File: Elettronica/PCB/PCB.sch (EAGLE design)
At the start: 60 parts, among them IC1 7805TV, J2 455-1750-1-ND, SW2 EC12E_SW

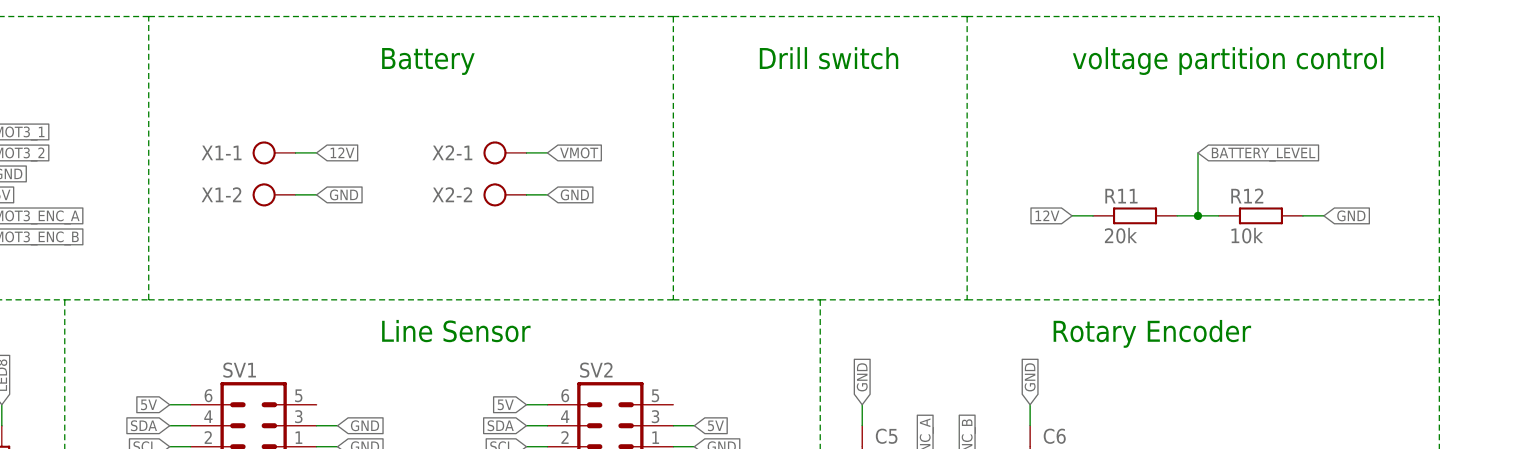
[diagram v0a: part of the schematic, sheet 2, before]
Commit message: PCB schematico
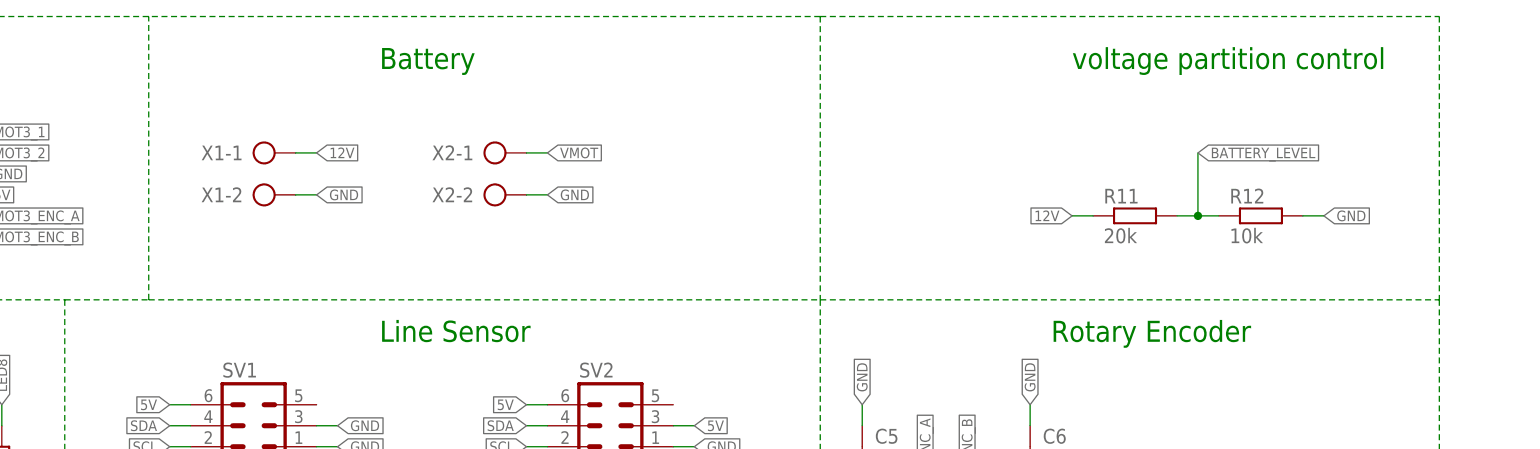
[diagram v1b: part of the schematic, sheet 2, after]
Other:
- note removed: "Drill switch"
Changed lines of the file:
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@@
 <?xml version="1.0" encoding="utf-8"?>
 <!DOCTYPE eagle SYSTEM "eagle.dtd">
-<eagle version="9.3.1">
+<eagle version="9.2.2">
 <drawing>
 <settings>
@@
 <text x="40.64" y="167.64" size="2.54" layer="91">Encoder pin</text>
 <text x="127" y="167.64" size="2.54" layer="91">Battery</text>
-<text x="172.72" y="167.64" size="2.54" layer="91">Drill switch</text>
 <text x="43.18" y="134.62" size="2.54" layer="91">Led</text>
 <text x="121.92" y="109.22" size="1.778" layer="91">ADR-GND
@@
 <wire x1="160.02" y1="5.08" x2="160.02" y2="25.4" width="1.016" layer="91" style="longdash"/>
 <wire x1="160.02" y1="25.4" x2="255.27" y2="25.4" width="1.016" layer="91" style="longdash"/>
-<wire x1="198.12" y1="173.99" x2="162.56" y2="173.99" width="1.016" layer="91" style="longdash"/>
-<wire x1="162.56" y1="173.99" x2="99.06" y2="173.99" width="1.016" layer="91" style="longdash"/>
+<wire x1="180.34" y1="173.99" x2="99.06" y2="173.99" width="1.016" layer="91" style="longdash"/>
 <wire x1="99.06" y1="173.99" x2="5.08" y2="173.99" width="1.016" layer="91" style="longdash"/>
 <wire x1="5.08" y1="173.99" x2="5.08" y2="139.7" width="1.016" layer="91" style="longdash"/>
@@
 <wire x1="88.9" y1="139.7" x2="99.06" y2="139.7" width="1.016" layer="91" style="longdash"/>
 <wire x1="99.06" y1="139.7" x2="99.06" y2="173.99" width="1.016" layer="91" style="longdash"/>
-<wire x1="99.06" y1="139.7" x2="162.56" y2="139.7" width="1.016" layer="91" style="longdash"/>
-<wire x1="162.56" y1="139.7" x2="180.34" y2="139.7" width="1.016" layer="91" style="longdash"/>
-<wire x1="180.34" y1="139.7" x2="198.12" y2="139.7" width="1.016" layer="91" style="longdash"/>
-<wire x1="198.12" y1="173.99" x2="198.12" y2="139.7" width="1.016" layer="91" style="longdash"/>
-<wire x1="162.56" y1="173.99" x2="162.56" y2="139.7" width="1.016" layer="91" style="longdash"/>
+<wire x1="99.06" y1="139.7" x2="180.34" y2="139.7" width="1.016" layer="91" style="longdash"/>
+<wire x1="180.34" y1="173.99" x2="180.34" y2="139.7" width="1.016" layer="91" style="longdash"/>
 <wire x1="5.08" y1="88.9" x2="50.8" y2="88.9" width="1.016" layer="91" style="longdash"/>
 <wire x1="50.8" y1="88.9" x2="88.9" y2="88.9" width="1.016" layer="91" style="longdash"/>
@@
 <wire x1="104.14" y1="22.86" x2="104.14" y2="38.1" width="1.016" layer="91" style="longdash"/>
 <wire x1="104.14" y1="38.1" x2="104.14" y2="60.96" width="1.016" layer="91" style="longdash"/>
-<wire x1="198.12" y1="173.99" x2="255.27" y2="173.99" width="1.016" layer="91" style="longdash"/>
+<wire x1="180.34" y1="173.99" x2="255.27" y2="173.99" width="1.016" layer="91" style="longdash"/>
 <wire x1="255.27" y1="173.99" x2="255.27" y2="139.7" width="1.016" layer="91" style="longdash"/>
 <wire x1="255.27" y1="139.7" x2="255.27" y2="88.9" width="1.016" layer="91" style="longdash"/>
 <wire x1="255.27" y1="88.9" x2="255.27" y2="60.96" width="1.016" layer="91" style="longdash"/>
 <wire x1="255.27" y1="60.96" x2="255.27" y2="25.4" width="1.016" layer="91" style="longdash"/>
-<wire x1="198.12" y1="139.7" x2="255.27" y2="139.7" width="1.016" layer="91" style="longdash"/>
+<wire x1="180.34" y1="139.7" x2="255.27" y2="139.7" width="1.016" layer="91" style="longdash"/>
 <wire x1="180.34" y1="88.9" x2="255.27" y2="88.9" width="1.016" layer="91" style="longdash"/>
 <wire x1="111.76" y1="60.96" x2="142.24" y2="60.96" width="1.016" layer="91" style="longdash"/>
